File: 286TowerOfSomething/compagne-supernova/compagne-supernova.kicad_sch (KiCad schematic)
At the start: 18 parts, among them J1 Bus_ISA_8bit, J2 DE9_Plug_MountingHoles, J3 DE9_Plug_MountingHoles, SW1 SW_DIP_x04, U1 16550, U2 GD75232N, U3 74HCU04, U4 74LS138, U5 74LS138, U6 16550, U7 GD75232N, U8 ATmega328PB-A, Y1 1.8432MHz

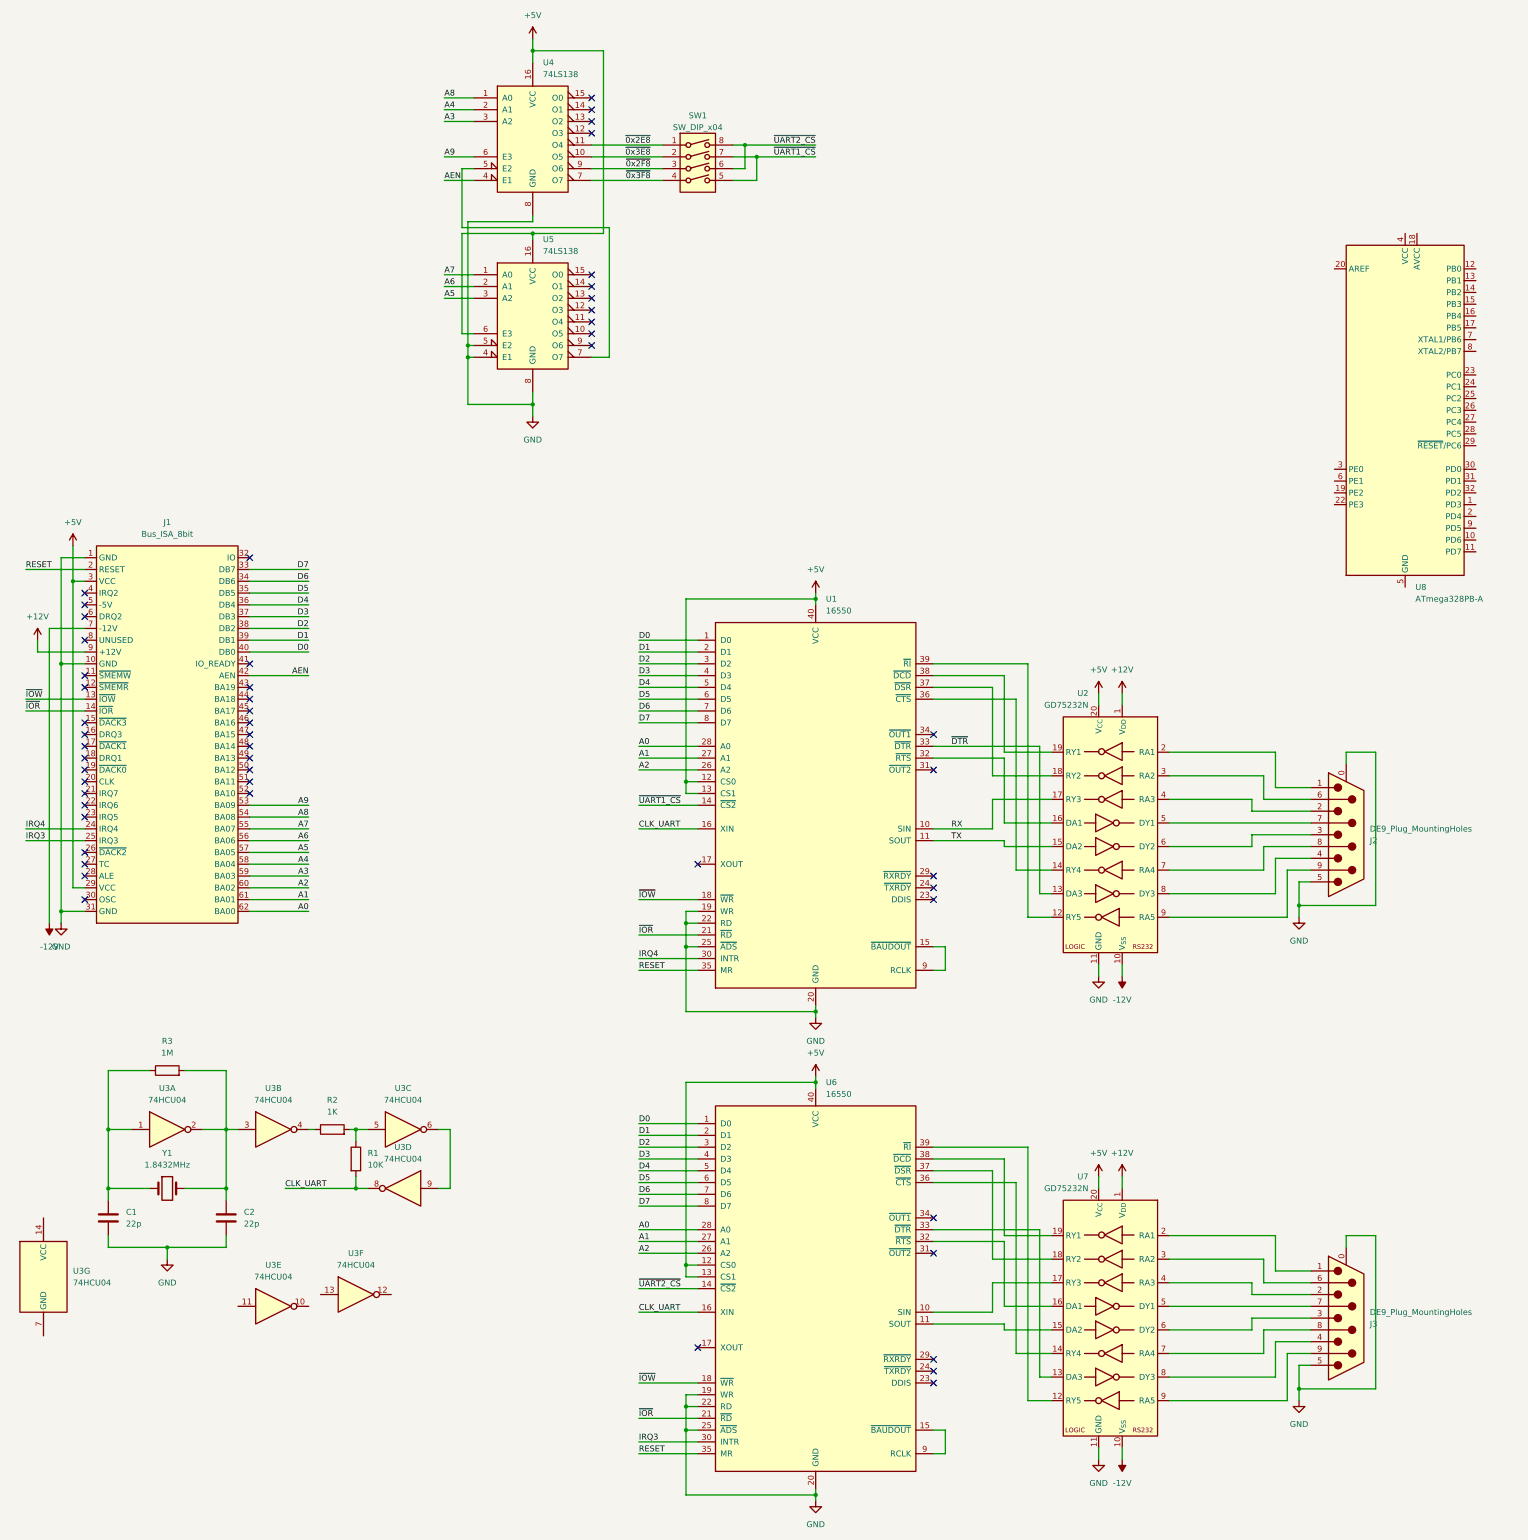
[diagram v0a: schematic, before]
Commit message: Finished schematic of compagne-supernova. Started messing with layout.
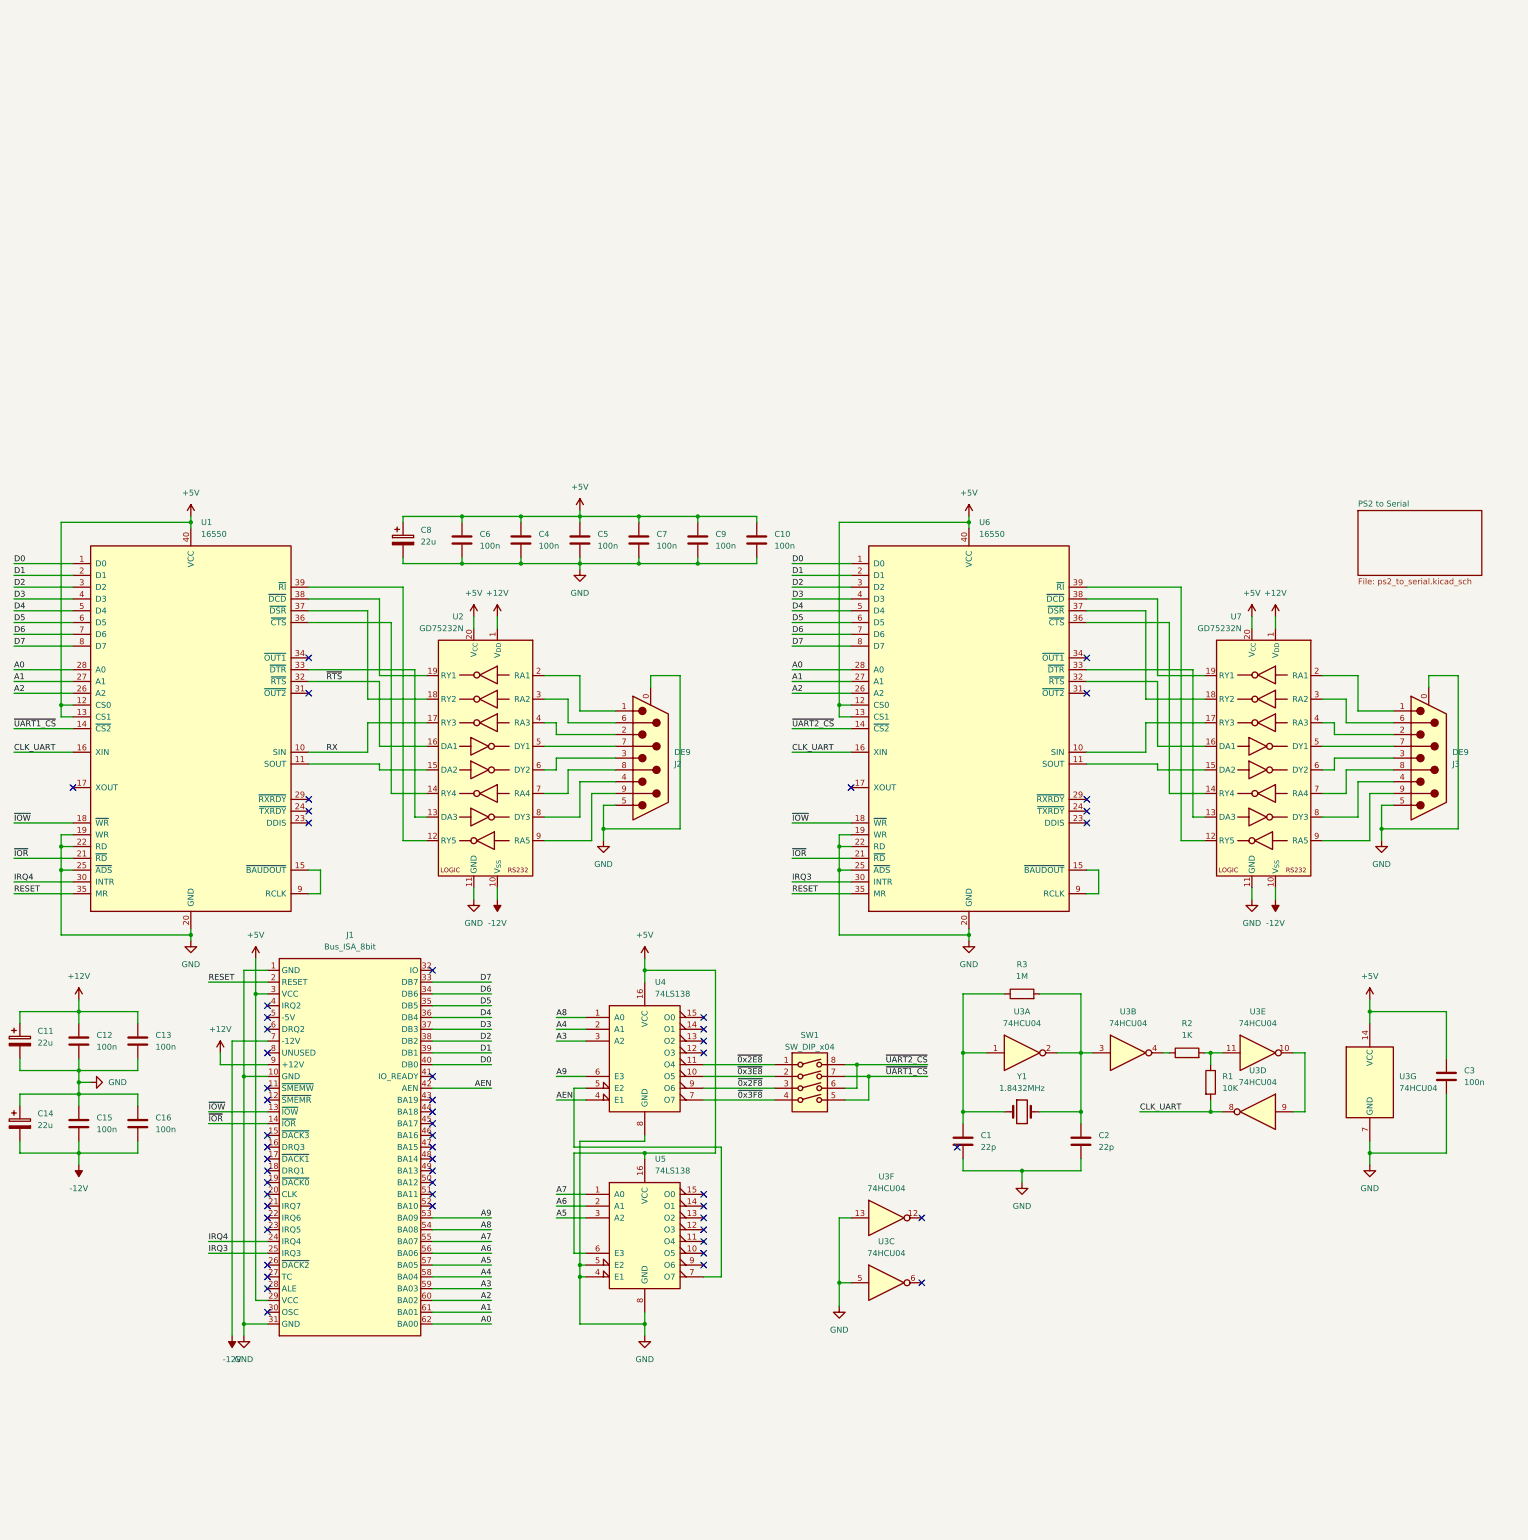
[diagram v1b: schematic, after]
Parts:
- removed U8: ATmega328PB-A, Package_QFP:TQFP-32_7x7mm_P0.8mm, symbol MCU_Microchip_ATmega:ATmega328PB-A
- added C10, C12, C13, C15, C16, C3, C4, C5, C6, C7, C9: 100n, Capacitor_SMD:C_0603_1608Metric_Pad1.08x0.95mm_HandSolder, symbol Device:C
- added C11, C14, C8: 22u, Capacitor_SMD:CP_Elec_5x5.3, symbol Device:C_Polarized
- C1, C2: footprint (none) -> Capacitor_SMD:C_0603_1608Metric_Pad1.08x0.95mm_HandSolder
- J1: footprint (none) -> pc-parts:BUS_AT_8BIT
- J2, J3: value DE9_Plug_MountingHoles -> DE9; footprint (none) -> Connector_Dsub:DSUB-9_Male_Horizontal_P2.77x2.84mm_EdgePinOffset7.70mm_Housed_MountingHolesOffset9.12mm
- R1, R2, R3: footprint (none) -> Resistor_SMD:R_0603_1608Metric_Pad0.98x0.95mm_HandSolder
- SW1: footprint (none) -> Button_Switch_THT:SW_DIP_SPSTx04_Slide_9.78x12.34mm_W7.62mm_P2.54mm
- U3: footprint (none) -> Package_SO:SO-14_3.9x8.65mm_P1.27mm
- U4, U5: footprint (none) -> Package_DIP:DIP-16_W7.62mm
- Y1: footprint (none) -> Crystal:Crystal_HC49-U_Vertical
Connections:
- net +12V: now also C11.1, C12.1, C13.1
- net +5V: now also U3.14 (VCC), C10.1, C3.1, C4.1, C5.1, C6.1, C7.1, C8.1, C9.1
- net -12V: now also C14.2, C15.2, C16.2
- net GND: now also U3.13, U3.5, U3.7 (GND), C10.2, C11.2, C12.2, C13.2, C14.1, C15.1, C16.1, C3.2, C4.2, C5.2, C6.2, C7.2, C8.2, C9.2
- net at U3.9: now also U3.10; no longer U3.6
- net at R1.1, R2.2: now also U3.11; no longer U3.5
- net ~{RTS}: now reaches U1.32 (~{RTS}), U2.16 (DA1)
- net TX: no longer names the net of U1.11 (SOUT), U2.15 (DA2)
- net ~{DTR}: no longer names the net of U1.33 (~{DTR}), U2.13 (DA3)
- no-connect marks 54 -> 57
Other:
- added sheet PS2 to Serial (ps2_to_serial.kicad_sch)
- company: (none) -> Surreality Labs
- title: (none) -> COMpagne Supernova
- moved on the sheet: C1, C2, J1, J2, J3, R1, R2, R3, SW1, U1, U2, U3A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
